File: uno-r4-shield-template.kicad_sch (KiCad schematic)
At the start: 52 parts, among them J1 POWER1, J10 +5V output, J11 +3.3V output, J12 Solder Pads 2, J13 GND, J14 Pin17 Rasp Pi LED Green, J15 Pilot Lamp Buzzer, J16 220VAC Detection In, J17 220VAC Detection Out, J19 GSM LED, J2 ANALOG, J20 Rasp Pi Control, J3 GSM LED Orange, J4 DIGITAL2, J5 DIGITAL1, J6 Pin8 Arduino LED Blue, J7 +12V Input, J8 Bill Acceptor, J9 Coin Acceptor, K1 G5LE-1-DC5, K2 G5LE-1-DC5, K3 G5LE-1-DC5, Q1 BC337, Q2 BC337, Q3 BC337, U1 DCDC_StepDown_LM2596, U2 EL817, U3 EL817, U4 EL817

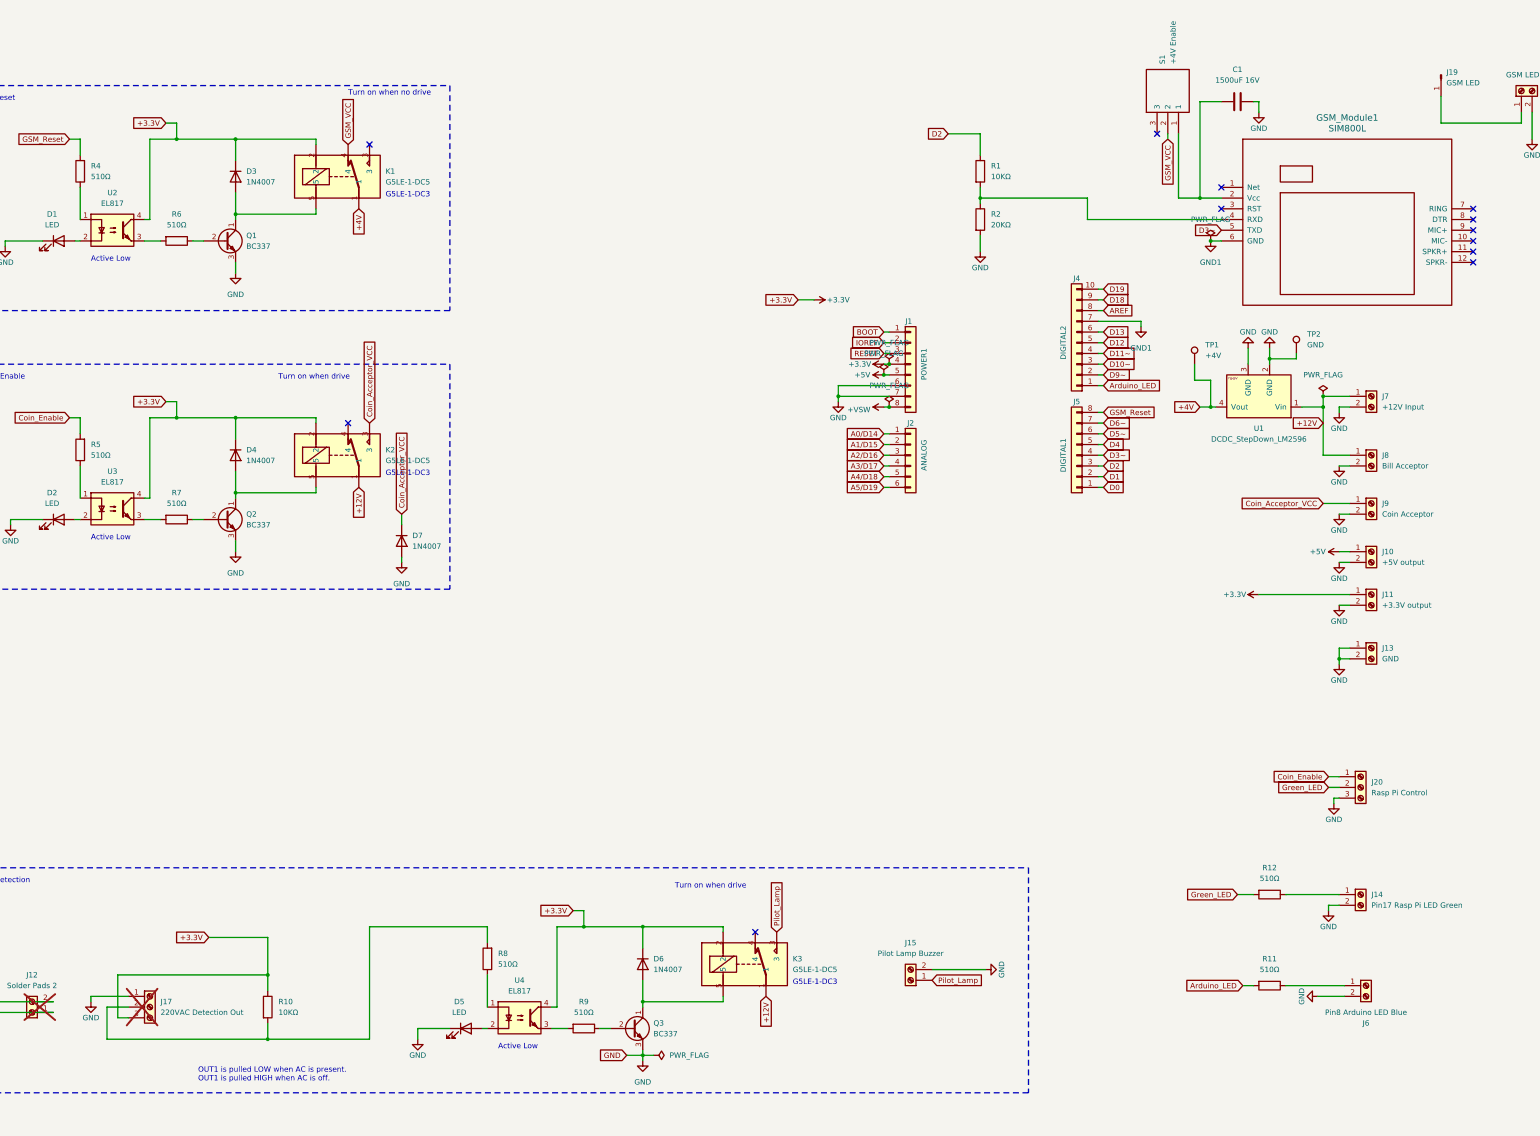
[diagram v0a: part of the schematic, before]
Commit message: Add files via upload
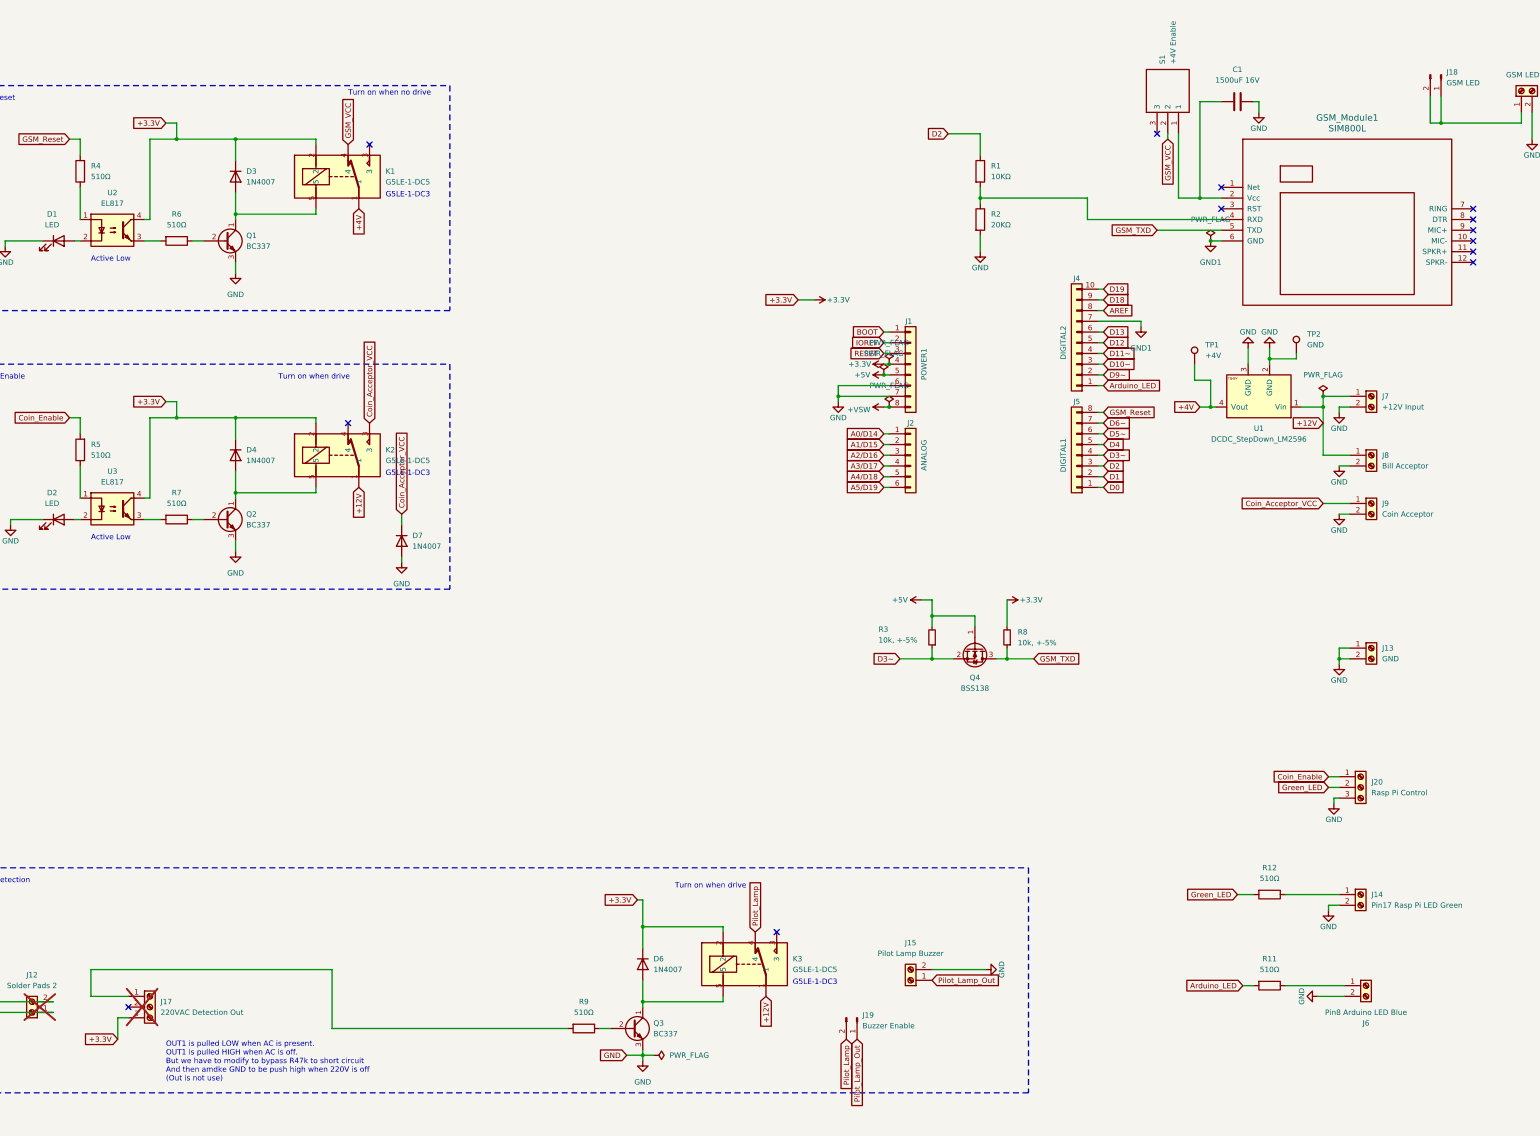
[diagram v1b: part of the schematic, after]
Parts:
- removed D5: LED, LED_THT:LED_D3.0mm, symbol Device:LED
- removed J10: +5V output, TerminalBlock_Phoenix:TerminalBlock_Phoenix_MKDS-1,5-2-5.08_1x02_P5.08mm_Horizontal, symbol Connector:Screw_Terminal_01x02
- removed J11: +3.3V output, TerminalBlock_Phoenix:TerminalBlock_Phoenix_MKDS-1,5-2-5.08_1x02_P5.08mm_Horizontal, symbol Connector:Screw_Terminal_01x02
- removed J19: GSM LED, Connector_PinHeader_2.54mm:PinHeader_1x01_P2.54mm_Vertical, symbol Connector:Conn_01x01_Pin
- removed R10: 10KΩ, Resistor_THT:R_Axial_DIN0207_L6.3mm_D2.5mm_P10.16mm_Horizontal, symbol Device:R
- removed R8: 510Ω, Resistor_THT:R_Axial_DIN0207_L6.3mm_D2.5mm_P10.16mm_Horizontal, symbol Device:R
- removed U4: EL817, Package_DIP:DIP-4_W7.62mm, symbol Isolator:EL817
- added J18: GSM LED, Connector_PinHeader_2.54mm:PinHeader_1x02_P2.54mm_Vertical, symbol Connector:Conn_01x02_Pin
- added J19: Buzzer Enable, Connector_PinHeader_2.54mm:PinHeader_1x02_P2.54mm_Vertical, symbol Connector:Conn_01x02_Pin
- added Q4: BSS138, Package_TO_SOT_SMD:SOT-23, symbol Transistor_FET:BSS138
- added R3, R8: 10k, +-5%, Resistor_THT:R_Axial_DIN0204_L3.6mm_D1.6mm_P5.08mm_Horizontal, symbol Device:R_Small
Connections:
- net +3V3: now also R8.2
- net +5V: now also Q4.1 (G), R3.2
- net D3~: now also Q4.2 (S), R3.1; no longer GSM_Module1.5 (TXD)
- net GND: no longer J17.1 (Pin_1)
- net Pilot_Lamp: now also K3.4, J19.2 (Pin_2); no longer J15.1 (Pin_1), K3.3
- net at J3.1 (Pin_1): now also J18.1 (Pin_1), J18.2 (Pin_2)
- net at R9.2: now also J17.1 (Pin_1)
- new net GSM_TXD: GSM_Module1.5 (TXD), Q4.3 (D), R8.1
- new net Pilot_Lamp_Out: J15.1 (Pin_1), J19.1 (Pin_1)
- no-connect marks 12 -> 13
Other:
- note added: "OUT1 is pulled LOW when AC is present. OUT1 is pulled HIGH when AC is off. But we have to modify to bypass R47k to short circuit And then amdke GND to be push high when 220V is off (Out is not use)"
- note removed: "OUT1 is pulled LOW when AC is present. OUT1 is pulled HIGH when AC is off."
